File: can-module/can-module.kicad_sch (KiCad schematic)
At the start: 26 parts, among them IC1 PIC32CM1216JH01048-I_U5B, J1 Conn_01x04_Socket, J2 Conn_01x04_Socket, J3 Conn_01x04_Socket, U1 ATA6560-GBQW-N

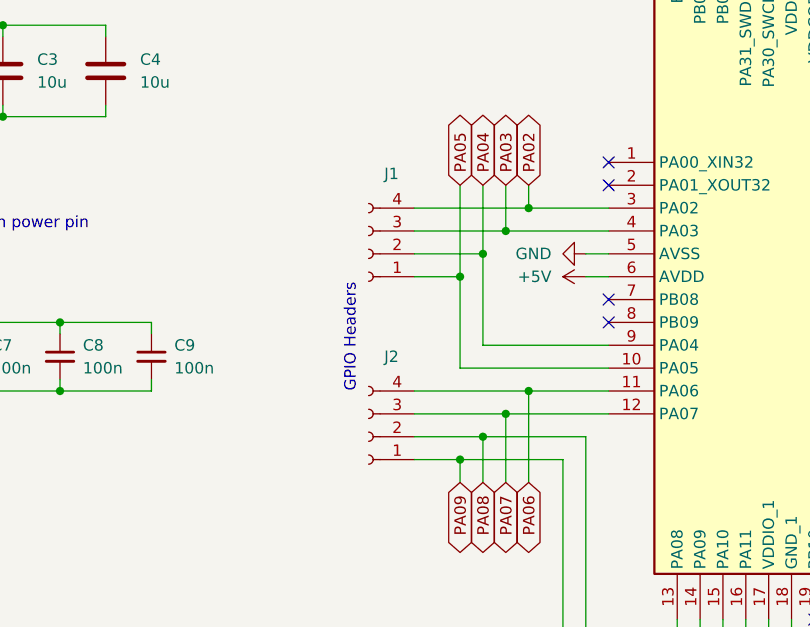
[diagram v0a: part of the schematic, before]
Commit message: can-module: Convert GPIO header from 2x 4pin header to 1x 8pin
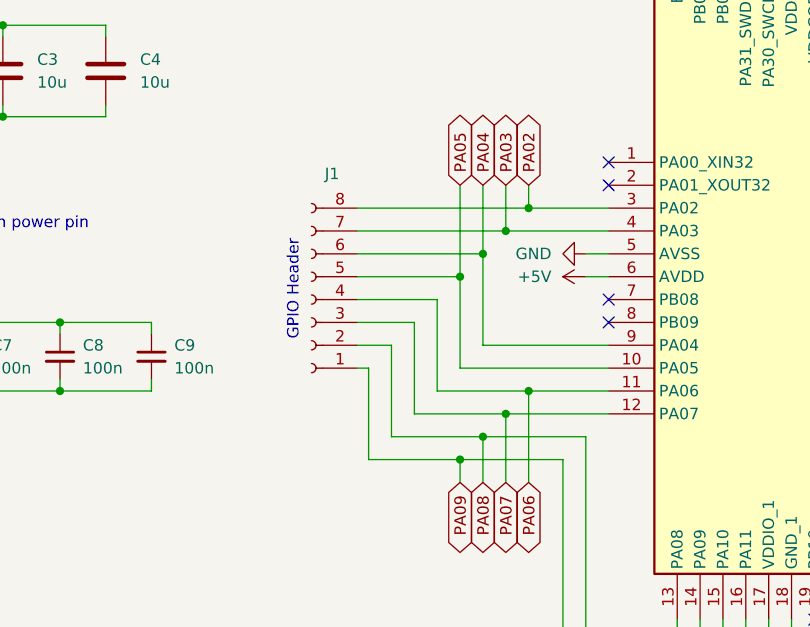
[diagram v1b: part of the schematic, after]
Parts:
- removed J1, J2: Conn_01x04_Socket, Conn01x04:01x04_1mm, symbol Connector:Conn_01x04_Socket
- added J1: Conn_01x08_Socket, Conn_01x08:Untitled, symbol Connector:Conn_01x08_Socket
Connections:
- net PA02: now also J1.8 (Pin_8)
- net PA03: now also J1.7 (Pin_7)
- net PA04: now also J1.6 (Pin_6)
- net PA05: now also J1.5 (Pin_5)
- net PA06: now also J1.4 (Pin_4)
- net PA07: now also J1.3 (Pin_3)
- net PA08: now also J1.2 (Pin_2)
- net PA09: now also J1.1 (Pin_1)
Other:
- note added: "GPIO Header"
- note removed: "GPIO Headers"

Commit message: can-module: Update PCB to match requirements for JLCPCB economic PCBA
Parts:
- C10, C11, C5, C6, C7, C8, C9: footprint Capacitor_SMD:C_0201_0603Metric -> Capacitor_SMD:C_0402_1005Metric
- R1, R2, R3: footprint Resistor_SMD:R_0201_0603Metric -> Resistor_SMD:R_0402_1005Metric
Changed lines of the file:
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@@
 			)
 		)
-		(property "Footprint" "Capacitor_SMD:C_0201_0603Metric"
+		(property "Footprint" "Capacitor_SMD:C_0402_1005Metric"
 			(at 69.85 123.19 0)
 			(effects
@@
 			)
 		)
-		(property "Footprint" "Capacitor_SMD:C_0201_0603Metric"
+		(property "Footprint" "Capacitor_SMD:C_0402_1005Metric"
 			(at 170.18 69.85 0)
 			(effects
@@
 			)
 		)
-		(property "Footprint" "Resistor_SMD:R_0201_0603Metric"
+		(property "Footprint" "Resistor_SMD:R_0402_1005Metric"
 			(at 170.18 62.23 0)
 			(effects
@@
 			)
 		)
-		(property "Footprint" "Capacitor_SMD:C_0201_0603Metric"
+		(property "Footprint" "Capacitor_SMD:C_0402_1005Metric"
 			(at 276.86 113.03 0)
 			(effects
@@
 			)
 		)
-		(property "Footprint" "Capacitor_SMD:C_0201_0603Metric"
+		(property "Footprint" "Capacitor_SMD:C_0402_1005Metric"
 			(at 59.69 123.19 0)
 			(effects
@@
 			)
 		)
-		(property "Footprint" "Capacitor_SMD:C_0201_0603Metric"
+		(property "Footprint" "Capacitor_SMD:C_0402_1005Metric"
 			(at 49.53 123.19 0)
 			(effects
@@
 			)
 		)
-		(property "Footprint" "Resistor_SMD:R_0201_0603Metric"
+		(property "Footprint" "Resistor_SMD:R_0402_1005Metric"
 			(at 142.24 53.34 0)
 			(effects
@@
 			)
 		)
-		(property "Footprint" "Resistor_SMD:R_0201_0603Metric"
+		(property "Footprint" "Resistor_SMD:R_0402_1005Metric"
 			(at 235.458 49.53 90)
 			(effects
@@
 			)
 		)
-		(property "Footprint" "Capacitor_SMD:C_0201_0603Metric"
+		(property "Footprint" "Capacitor_SMD:C_0402_1005Metric"
 			(at 39.37 123.19 0)
 			(effects
@@
 			)
 		)
-		(property "Footprint" "Capacitor_SMD:C_0201_0603Metric"
+		(property "Footprint" "Capacitor_SMD:C_0402_1005Metric"
 			(at 29.21 123.19 0)
 			(effects
